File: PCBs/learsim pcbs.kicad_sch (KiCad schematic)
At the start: 52 parts, among them J1 +5V_IN, SW1 MHz, SW2 KHz, U1 ESP32-C6-DEV-KIT-N8, U2 MAX7219, U3 MAX7219

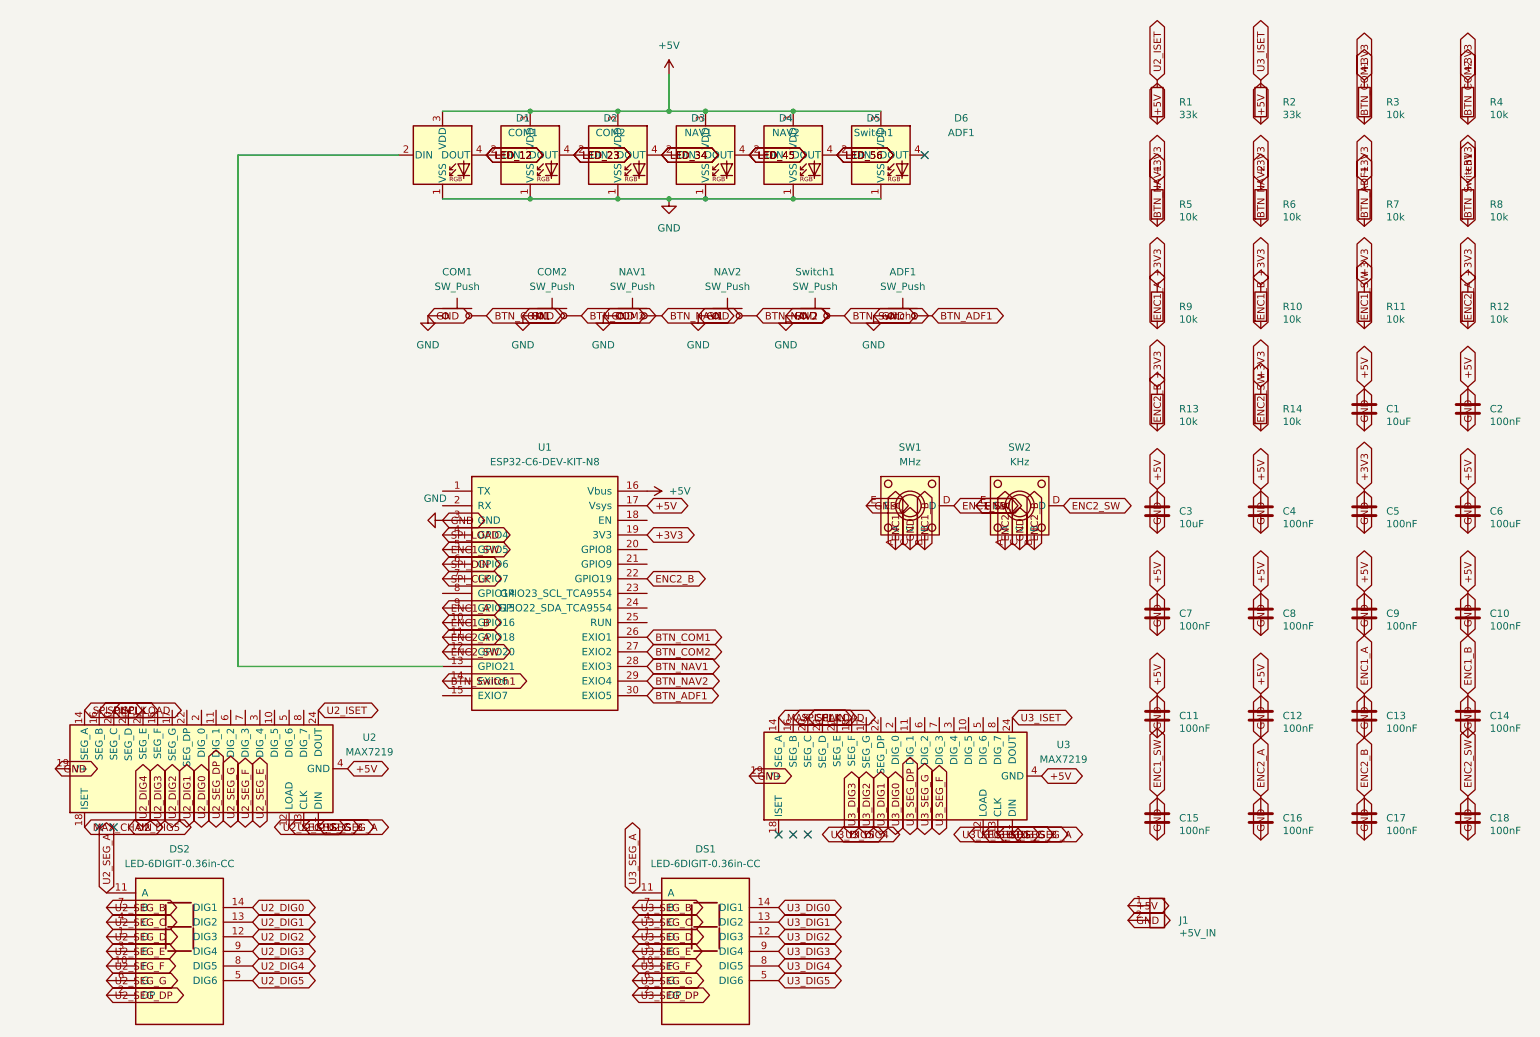
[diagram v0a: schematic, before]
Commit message: Refactor code structure for improved readability and maintainability
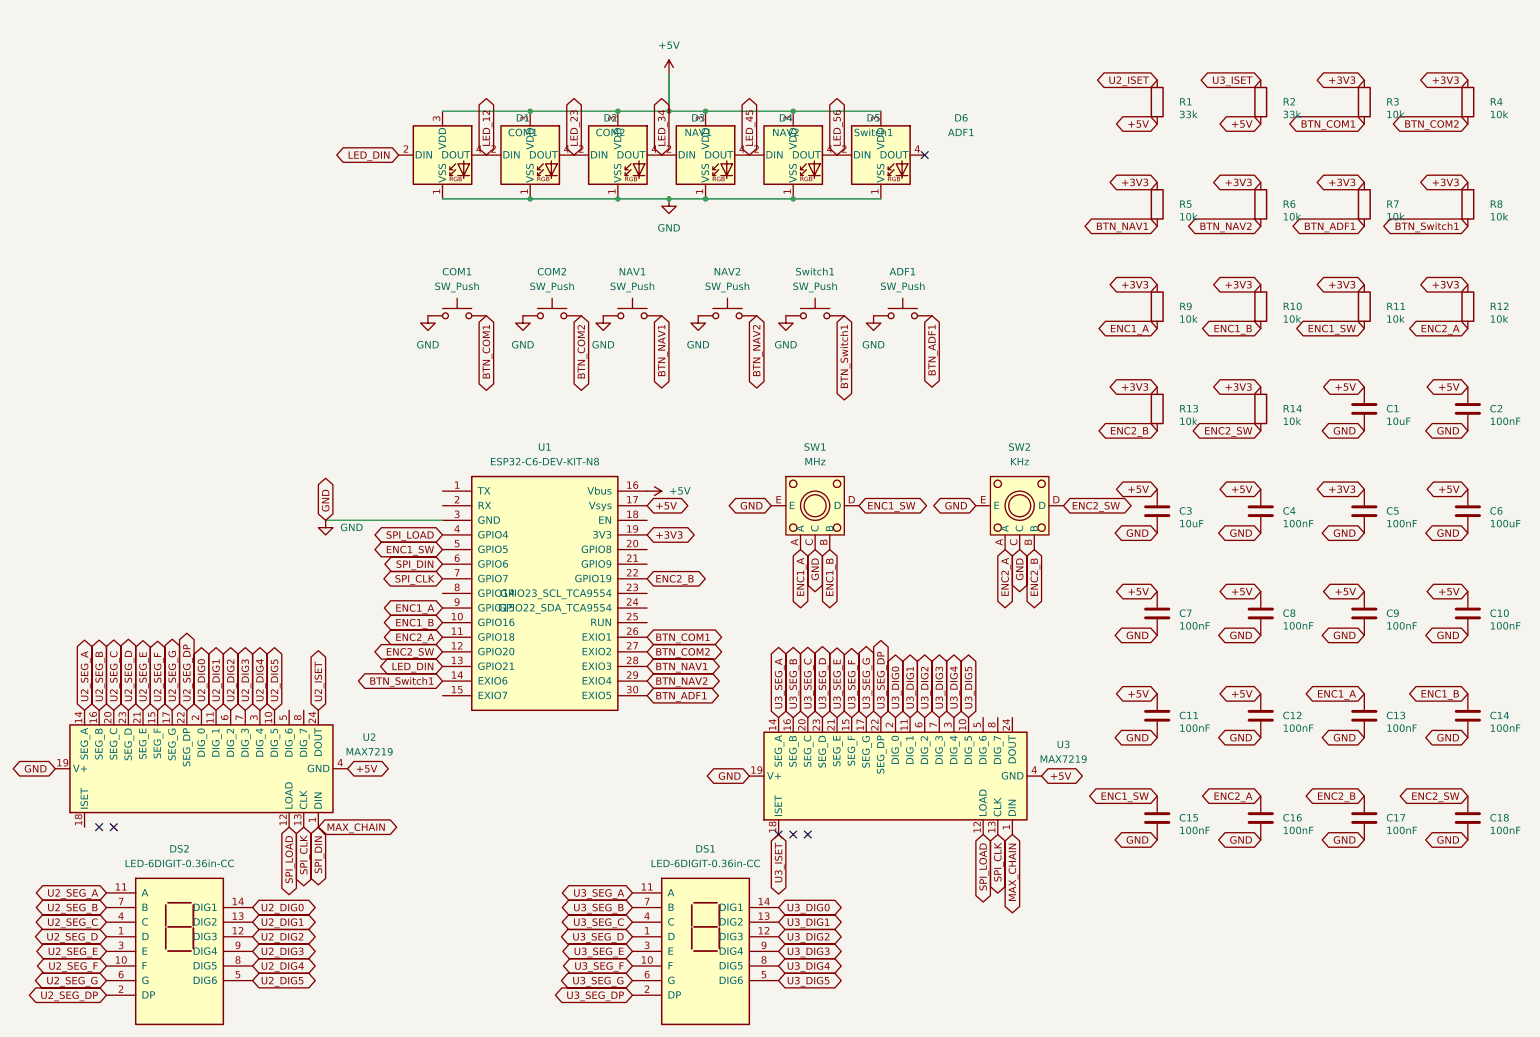
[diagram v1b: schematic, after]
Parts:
- removed J1: +5V_IN, TerminalBlock:TerminalBlock_bornier-2_P5.08mm, symbol Connector:Screw_Terminal_01x02
- DS1, DS2: footprint LED-6DIGIT-0.36in-CC_14P:LED-6DIGIT-0.36in-CC_14P -> 7-Segment Display:LED-6DIGIT-0.36in-CC_14P
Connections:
- net MAX_CHAIN: now also U1.6 (GPIO6), U2.1 (DIN), U3.1 (DIN); no longer U2.18 (ISET), U3.14 (SEG_A)
- net SPI_CLK: now also U2.13 (CLK), U3.13 (CLK); no longer U2.16 (SEG_B), U3.16 (SEG_B)
- net SPI_LOAD: now also U2.12 (LOAD), U3.12 (LOAD); no longer U2.20 (SEG_C), U3.20 (SEG_C)
- net U2_DIG0: now also U2.2 (DIG_0)
- net U2_DIG1: now also U2.11 (DIG_1)
- net U2_DIG2: now also U2.6 (DIG_2)
- net U2_DIG3: now also U2.7 (DIG_3)
- net U2_DIG4: now also U2.3 (DIG_4)
- net U2_DIG5: now also U2.10 (DIG_5)
- net U2_SEG_A: now also U2.14 (SEG_A); no longer U2.1 (DIN)
- net U2_SEG_B: now also U2.16 (SEG_B); no longer U2.13 (CLK)
- net U2_SEG_C: now also U2.20 (SEG_C); no longer U2.12 (LOAD)
- net U2_SEG_D: now also U2.23 (SEG_D)
- net U2_SEG_DP: now also U2.22 (SEG_DP)
- net U2_SEG_E: now also U2.21 (SEG_E)
- net U2_SEG_F: now also U2.15 (SEG_F)
- net U2_SEG_G: now also U2.17 (SEG_G)
- net U3_DIG0: now also U3.2 (DIG_0)
- net U3_DIG1: now also U3.11 (DIG_1)
- net U3_DIG2: now also U3.6 (DIG_2)
- net U3_DIG3: now also U3.7 (DIG_3)
- net U3_DIG4: now also U3.3 (DIG_4)
- net U3_DIG5: now also U3.10 (DIG_5)
- net U3_ISET: now also U3.18 (ISET); no longer U3.24 (DOUT)
- net U3_SEG_A: now also U3.14 (SEG_A); no longer U3.1 (DIN)
- net U3_SEG_B: now also U3.16 (SEG_B); no longer U3.13 (CLK)
- net U3_SEG_C: now also U3.20 (SEG_C); no longer U3.12 (LOAD)
- net U3_SEG_D: now also U3.23 (SEG_D)
- net U3_SEG_DP: now also U3.22 (SEG_DP)
- net U3_SEG_E: now also U3.21 (SEG_E)
- net U3_SEG_F: now also U3.15 (SEG_F)
- net U3_SEG_G: now also U3.17 (SEG_G)
- net LED_DIN: now reaches D1.2 (DIN), U1.13 (GPIO21)
- removed net SPI_DIN: U1.6 (GPIO6), U2.14 (SEG_A)
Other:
- moved on the sheet: SW1
